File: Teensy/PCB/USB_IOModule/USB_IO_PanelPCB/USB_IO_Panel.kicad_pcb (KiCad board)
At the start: 2 copper layers, 61 x 128 mm, 31 parts, among them J1 USB_B, J2 USB_A

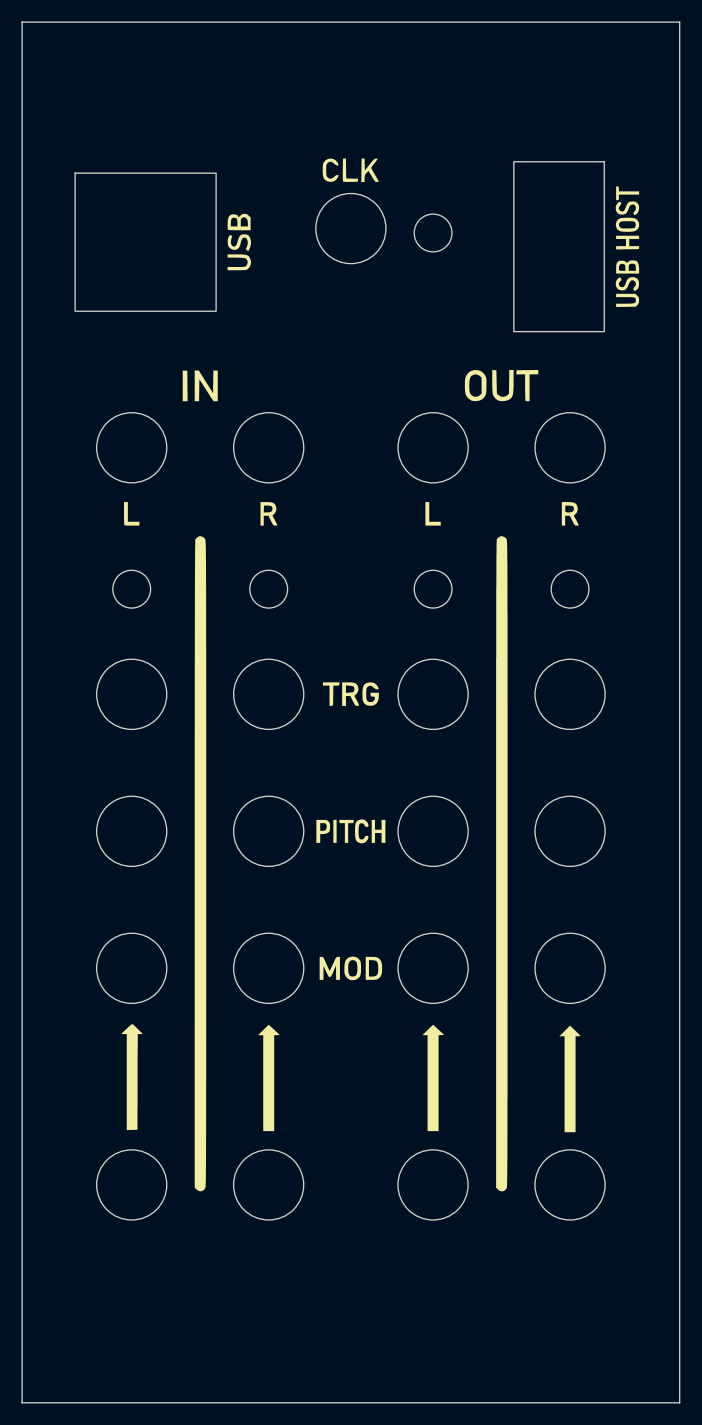
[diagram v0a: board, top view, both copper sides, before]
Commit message: Generated Gerbers
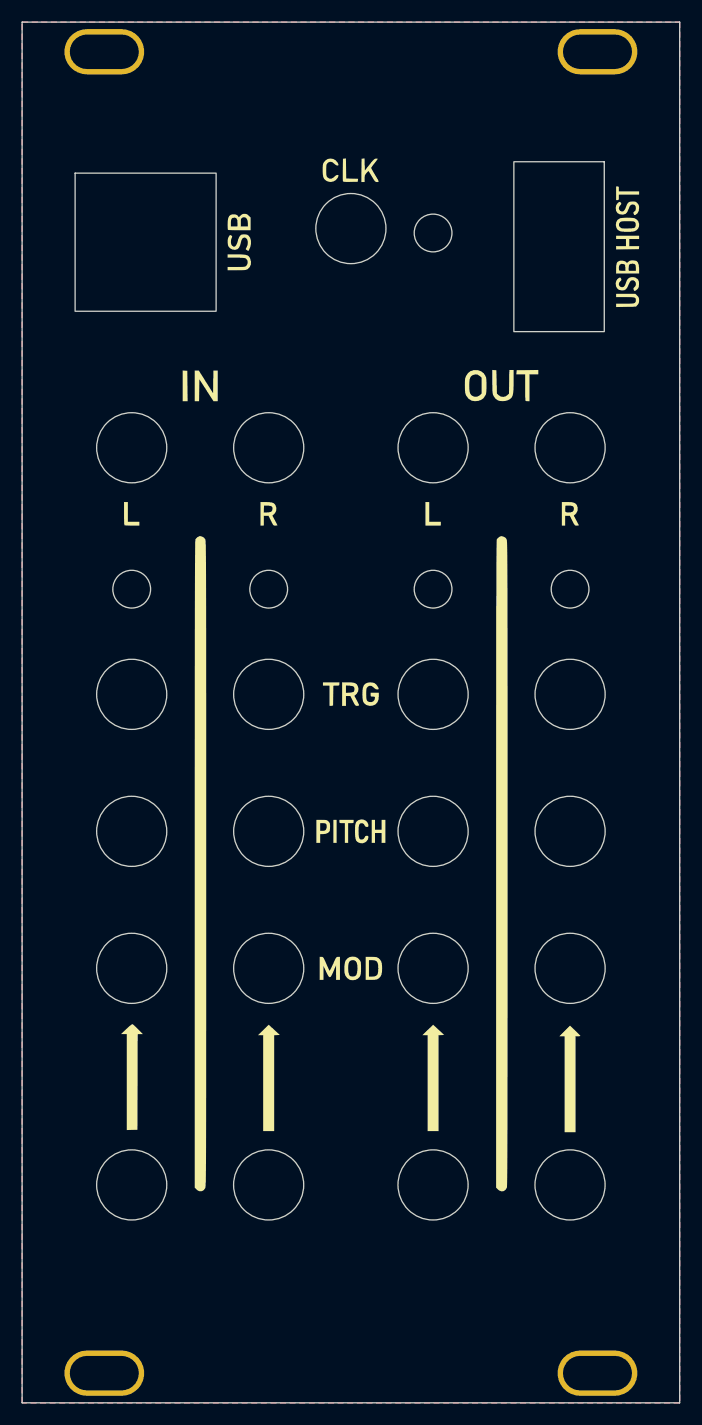
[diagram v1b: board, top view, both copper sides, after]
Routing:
- added copper zone on B.Cu, net shielding
- added copper zone on F.Cu, net shielding
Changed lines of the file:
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@@
       (layerselection 0x00010fc_ffffffff)
       (disableapertmacros false)
-      (usegerberextensions false)
-      (usegerberattributes true)
-      (usegerberadvancedattributes true)
-      (creategerberjobfile true)
+      (usegerberextensions true)
+      (usegerberattributes false)
+      (usegerberadvancedattributes false)
+      (creategerberjobfile false)
       (svguseinch false)
       (svgprecision 6)
@@
       (psa4output false)
       (plotreference true)
-      (plotvalue true)
+      (plotvalue false)
       (plotinvisibletext false)
       (sketchpadsonfab false)
-      (subtractmaskfromsilk false)
+      (subtractmaskfromsilk true)
       (outputformat 1)
       (mirror false)
-      (drillshape 1)
+      (drillshape 0)
       (scaleselection 1)
-      (outputdirectory "")
+      (outputdirectory "USB_IO_Panel_Gerber")
     )
   )
   (net 0 "")
+  (net 1 "shielding")
   (footprint "Potentiometer:Bourns_PTV09A-X_Hole" (layer "F.Cu")
     (at 91.435 157.48)
@@
     (fp_line (start -2.54 -64) (end 2.54 -64) (layer "User.1") (width 0.12))
     (fp_circle (center 0 0) (end 0 0) (layer "User.1") (width 0.12) (fill none))
-    (fp_line (start -1.27 -62.85) (end 1.27 -62.85) (layer "User.2") (width 0.12))
-    (fp_line (start -1.27 -59.65) (end 1.27 -59.65) (layer "User.2") (width 0.12))
-    (fp_line (start -1.27 59.65) (end 1.27 59.65) (layer "User.2") (width 0.12))
-    (fp_line (start -1.27 62.85) (end 1.27 62.85) (layer "User.2") (width 0.12))
-    (fp_arc (start -1.27 -59.65) (mid -2.87 -61.25) (end -1.27 -62.85) (layer "User.2") (width 0.12))
-    (fp_arc (start 1.27 59.65) (mid 2.87 61.25) (end 1.27 62.85) (layer "User.2") (width 0.12))
-    (fp_arc (start 1.27 -62.85) (mid 2.87 -61.25) (end 1.27 -59.65) (layer "User.2") (width 0.12))
-    (fp_arc (start -1.27 62.85) (mid -2.87 61.25) (end -1.27 59.65) (layer "User.2") (width 0.12))
-    (pad "" np_thru_hole oval (at 0 61.25) (size 5.74 3.2) (drill oval 5.74 3.2) (layers *.Mask))
-    (pad "" np_thru_hole oval (at 0 -61.25) (size 5.74 3.2) (drill oval 5.74 3.2) (layers *.Mask))
+    (fp_line (start -1.6 -59.65) (end 1.6 -59.65) (layer "User.2") (width 0.12))
+    (fp_line (start -1.6 62.85) (end 1.6 62.85) (layer "User.2") (width 0.12))
+    (fp_line (start -1.6 -62.85) (end 1.6 -62.85) (layer "User.2") (width 0.12))
+    (fp_line (start -1.6 59.65) (end 1.6 59.65) (layer "User.2") (width 0.12))
+    (fp_arc (start 1.6 -62.85) (mid 3.2 -61.25) (end 1.6 -59.65) (layer "User.2") (width 0.12))
+    (fp_arc (start -1.6 -59.65) (mid -3.2 -61.25) (end -1.6 -62.85) (layer "User.2") (width 0.12))
+    (fp_arc (start -1.6 62.85) (mid -3.2 61.25) (end -1.6 59.65) (layer "User.2") (width 0.12))
+    (fp_arc (start 1.6 59.65) (mid 3.2 61.25) (end 1.6 62.85) (layer "User.2") (width 0.12))
+    (pad "1" thru_hole oval (at 0 -61.25) (size 7.4 4.2) (drill oval 6.4 3.2) (layers *.Cu *.Mask)
+      (net 1 "shielding"))
+    (pad "1" thru_hole oval (at 0 61.25) (size 7.4 4.2) (drill oval 6.4 3.2) (layers *.Cu *.Mask)
+      (net 1 "shielding"))
   )
   (footprint "Perfboard:3.5mm Jack Perfboard_Hole" (layer "F.Cu")
@@
       (effects (font (size 1 1) (thickness 0.15)))
     )
+    (fp_line (start -2.54 64) (end 2.54 64) (layer "User.1") (width 0.12))
     (fp_line (start -2.54 -64) (end 2.54 -64) (layer "User.1") (width 0.12))
-    (fp_line (start -2.54 64) (end 2.54 64) (layer "User.1") (width 0.12))
     (fp_circle (center 0 0) (end 0 0) (layer "User.1") (width 0.12) (fill none))
-    (fp_line (start -1.27 59.65) (end 1.27 59.65) (layer "User.2") (width 0.12))
-    (fp_line (start -1.27 -62.85) (end 1.27 -62.85) (layer "User.2") (width 0.12))
-    (fp_line (start -1.27 -59.65) (end 1.27 -59.65) (layer "User.2") (width 0.12))
-    (fp_line (start -1.27 62.85) (end 1.27 62.85) (layer "User.2") (width 0.12))
-    (fp_arc (start 1.27 -62.85) (mid 2.87 -61.25) (end 1.27 -59.65) (layer "User.2") (width 0.12))
-    (fp_arc (start -1.27 -59.65) (mid -2.87 -61.25) (end -1.27 -62.85) (layer "User.2") (width 0.12))
-    (fp_arc (start -1.27 62.85) (mid -2.87 61.25) (end -1.27 59.65) (layer "User.2") (width 0.12))
-    (fp_arc (start 1.27 59.65) (mid 2.87 61.25) (end 1.27 62.85) (layer "User.2") (width 0.12))
-    (pad "" np_thru_hole oval (at 0 -61.25) (size 5.74 3.2) (drill oval 5.74 3.2) (layers *.Mask))
-    (pad "" np_thru_hole oval (at 0 61.25) (size 5.74 3.2) (drill oval 5.74 3.2) (layers *.Mask))
+    (fp_line (start -1.6 59.65) (end 1.6 59.65) (layer "User.2") (width 0.12))
+    (fp_line (start -1.6 -59.65) (end 1.6 -59.65) (layer "User.2") (width 0.12))
+    (fp_line (start -1.6 62.85) (end 1.6 62.85) (layer "User.2") (width 0.12))
+    (fp_line (start -1.6 -62.85) (end 1.6 -62.85) (layer "User.2") (width 0.12))
+    (fp_arc (start -1.6 -59.65) (mid -3.2 -61.25) (end -1.6 -62.85) (layer "User.2") (width 0.12))
+    (fp_arc (start 1.6 59.65) (mid 3.2 61.25) (end 1.6 62.85) (layer "User.2") (width 0.12))
+    (fp_arc (start -1.6 62.85) (mid -3.2 61.25) (end -1.6 59.65) (layer "User.2") (width 0.12))
+    (fp_arc (start 1.6 -62.85) (mid 3.2 -61.25) (end 1.6 -59.65) (layer "User.2") (width 0.12))
+    (pad "1" thru_hole oval (at 0 61.25) (size 7.4 4.2) (drill oval 6.4 3.2) (layers *.Cu *.Mask)
+      (net 1 "shielding"))
+    (pad "1" thru_hole oval (at 0 -61.25) (size 7.4 4.2) (drill oval 6.4 3.2) (layers *.Cu *.Mask)
+      (net 1 "shielding"))
   )
   (footprint "Perfboard:3.5mm Jack Perfboard_Hole" (layer "F.Cu")
@@
   )
   (gr_rect (start 68.58 42.68) (end 129.54 170.68) (layer "Edge.Cuts") (width 0.1) (fill none))
+  (zone (net 1) (net_name "shielding") (layers F&B.Cu) (hatch edge 0.508)
+    (connect_pads yes (clearance 0.508))
+    (min_thickness 0.254) (filled_areas_thickness no)
+    (fill yes (thermal_gap 0.508) (thermal_bridge_width 0.508))
+    (polygon
+      (pts
+        (xy 129.54 170.688)
+        (xy 68.58 170.688)
+        (xy 68.58 42.672)
+        (xy 129.54 42.672)
+      )
+    )
+  )
 )
